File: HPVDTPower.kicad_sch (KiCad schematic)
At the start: 1 part

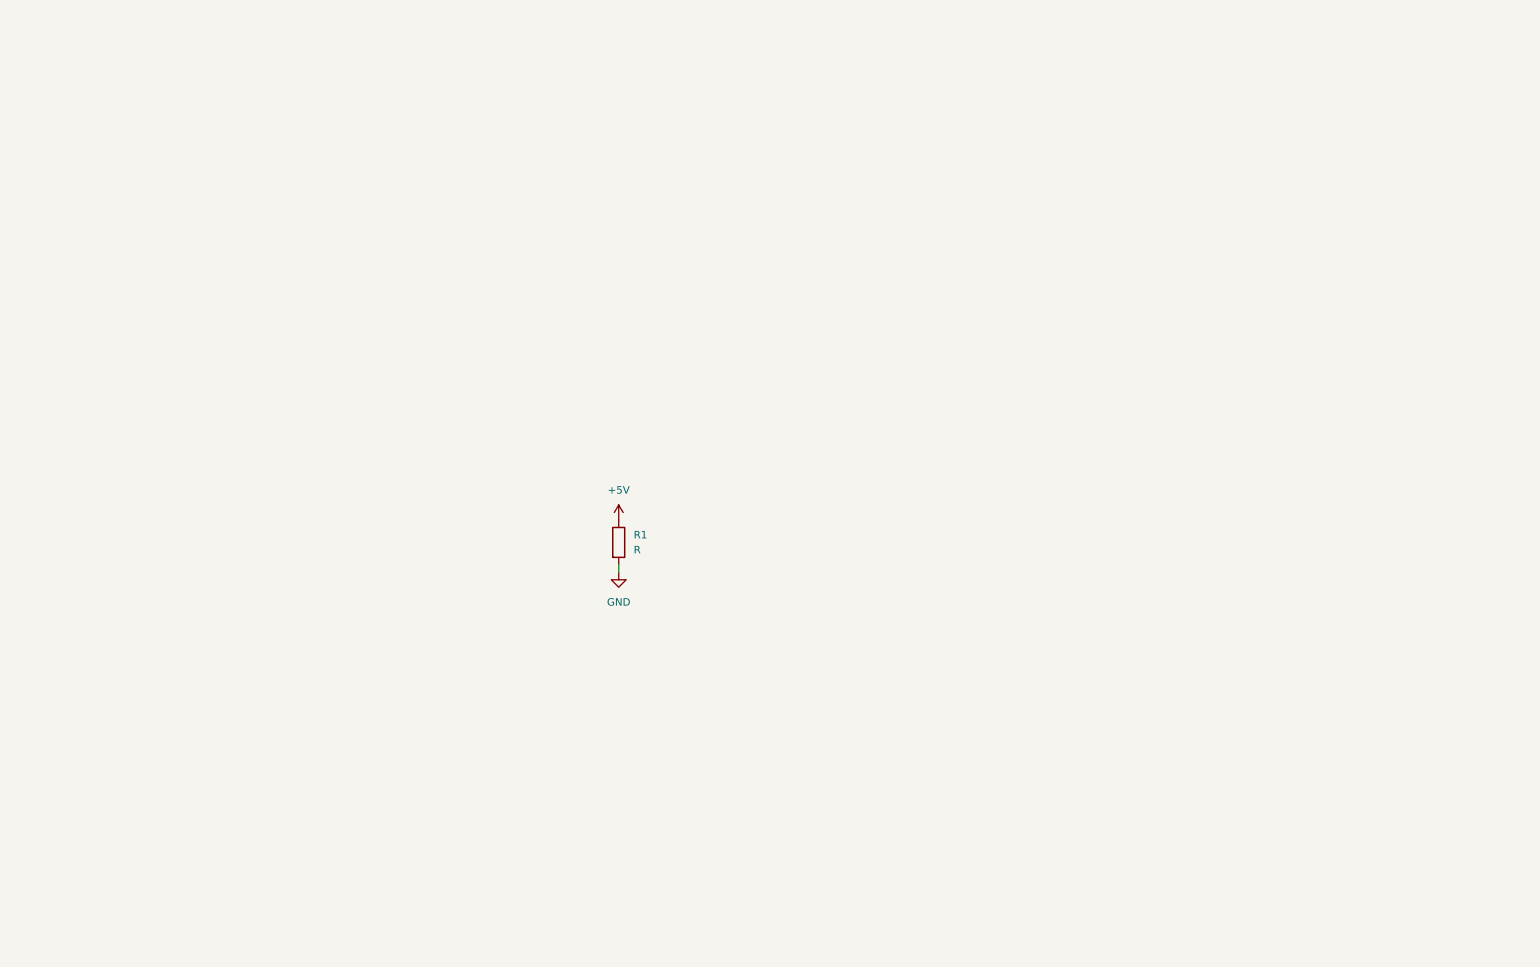
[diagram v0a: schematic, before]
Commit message: Update
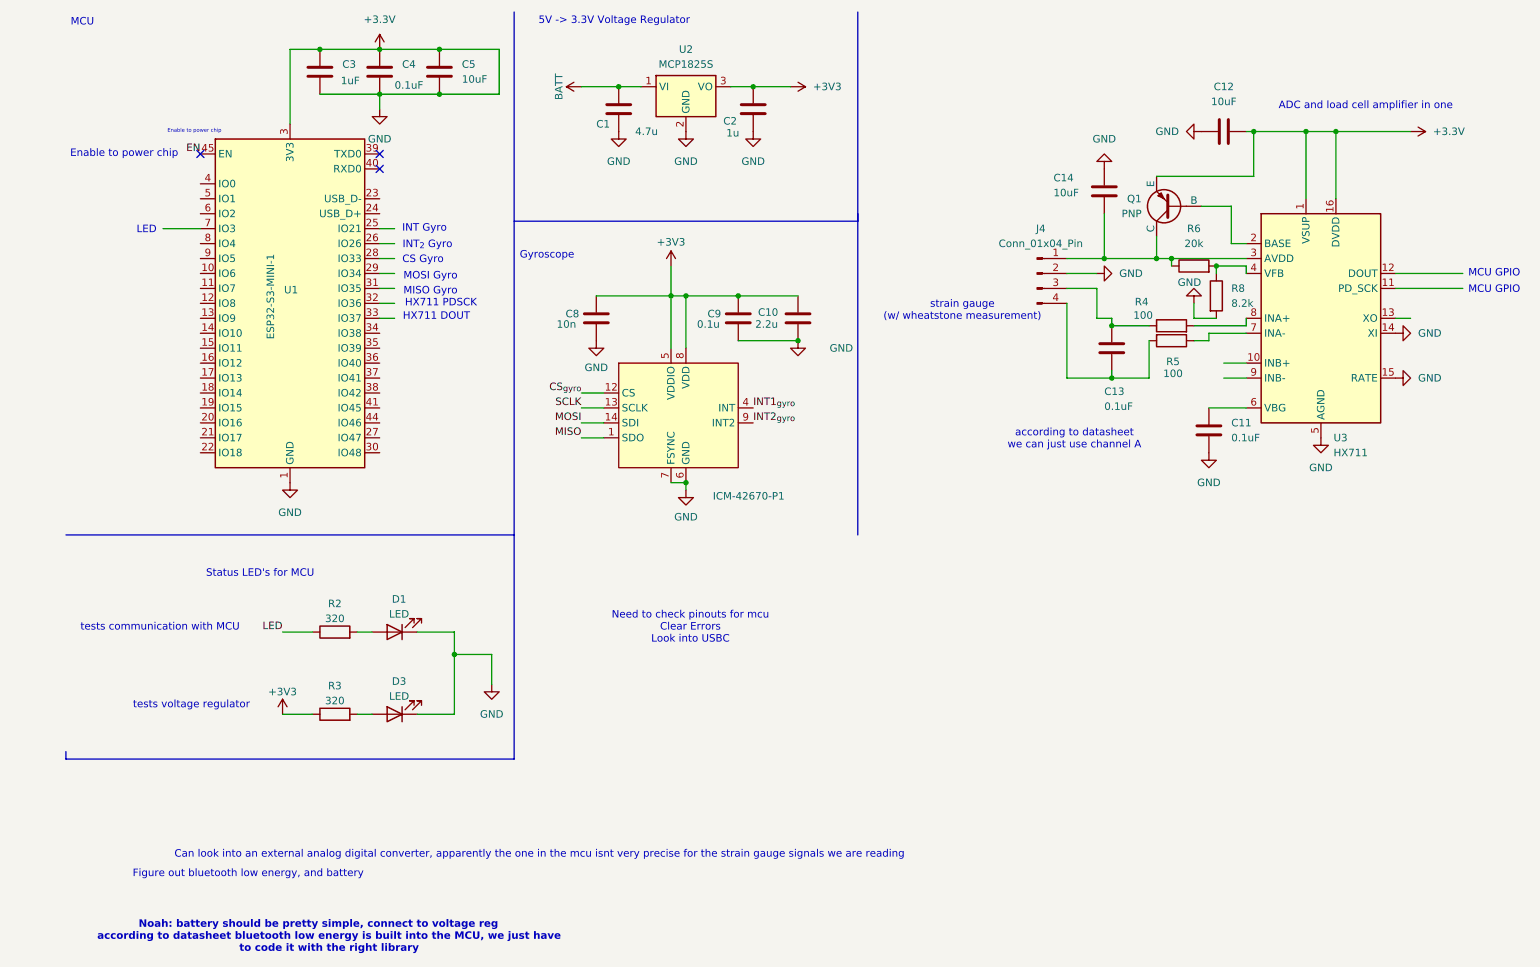
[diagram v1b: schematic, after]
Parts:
- removed R1: R, symbol Device:R
- added C1: 4.7u, Capacitor_SMD:C_0402_1005Metric, symbol Device:C
- added C10: 2.2u, Capacitor_SMD:C_0402_1005Metric, symbol Device:C
- added C11, C13, C4: 0.1uF, symbol Device:C
- added C12, C14, C5: 10uF, symbol Device:C
- added C2: 1u, Capacitor_SMD:C_0402_1005Metric, symbol Device:C
- added C3: 1uF, symbol Device:C
- added C8: 10n, Capacitor_SMD:C_0402_1005Metric, symbol Device:C
- added C9: 0.1u, Capacitor_SMD:C_0402_1005Metric, symbol Device:C
- added D1, D3: LED, LED_SMD:LED_0402_1005Metric, symbol Device:LED
- added ICM-42670-P1: ~, Package_LGA:LGA-14_3x2.5mm_P0.5mm_LayoutBorder3x4y, symbol 0_pwrmtr:ICM-42670-P
- added J4: Conn_01x04_Pin, Connector_JST:JST_EH_S4B-EH_1x04_P2.50mm_Horizontal, symbol Connector:Conn_01x04_Pin
- added Q1: PNP, symbol Simulation_SPICE:PNP
- added R2, R3: 320, Resistor_SMD:R_0402_1005Metric, symbol Device:R
- added R4, R5: 100, symbol Device:R
- added R6: 20k, symbol Device:R
- added R8: 8.2k, symbol Device:R
- added U1: ESP32-S3-MINI-1, RF_Module:ESP32-S2-MINI-1, symbol RF_Module:ESP32-S3-MINI-1
- added U2: MCP1825S, Package_TO_SOT_SMD:SOT-223-3_TabPin2, symbol Regulator_Linear:MCP1825S
- added U3: HX711, Package_SO:SOP-16_3.9x9.9mm_P1.27mm, symbol Analog_ADC:HX711
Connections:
- new net: D1.2 (A), R2.2
- new net: R5.1, U3.7 (INA-)
- new net: C13.2, J4.4 (Pin_4), R5.2
- new net: D3.2 (A), R3.2
- new net: C14.2, J4.1 (Pin_1), Q1.1 (C), R6.1, U3.3 (AVDD)
- new net: C13.1, J4.3 (Pin_3), R4.1
- new net: C11.1, U3.6 (VBG)
- new net: R6.2, R8.1, U3.4 (VFB)
- new net: R4.2, U3.8 (INA+)
- new net: Q1.2 (B), U3.2 (BASE)
- new net +3.3V: C1.1, C10.1, C11.2, C12.1, C12.2, C14.1, C2.1, C3.1, C3.2, C4.1, C4.2, C5.1, C5.2, C8.1, C9.1, D1.1 (K), D3.1 (K), ICM-42670-P1.6 (GND), ICM-42670-P1.7 (FSYNC), J4.2 (Pin_2), Q1.3 (E), R8.2, U1.1 (GND), U1.2 (GND), U1.3 (3V3), U1.42 (GND), U1.43 (GND), U1.46 (GND), U1.47 (GND), U1.48 (GND), U1.49 (GND), U1.50 (GND), U1.51 (GND), U1.52 (GND), U1.53 (GND), U1.54 (GND), U1.55 (GND), U1.56 (GND), U1.57 (GND), U1.58 (GND), U1.59 (GND), U1.60 (GND), U1.61 (GND), U1.62 (GND), U1.63 (GND), U1.64 (GND), U1.65 (GND), U2.2 (GND), U3.1 (VSUP), U3.14 (XI), U3.15 (RATE), U3.16 (DVDD), U3.5 (AGND)
- new net +3V3: C10.2, C2.2, C8.2, C9.2, ICM-42670-P1.5 (VDDIO), ICM-42670-P1.8 (VDD), R3.1, U2.3 (VO)
- new net BATT: C1.2, U2.1 (VI)
- new net CS_{gyro}: ICM-42670-P1.12 (CS)
- new net EN: U1.45 (EN)
- new net INT1_{gyro}: ICM-42670-P1.4 (INT)
- new net INT2_{gyro}: ICM-42670-P1.9 (INT2)
- new net LED: R2.1
- new net MISO: ICM-42670-P1.1 (SDO)
- new net MOSI: ICM-42670-P1.14 (SDI)
- new net SCLK: ICM-42670-P1.13 (SCLK)
- no-connect marks 0 -> 3
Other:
- note added: "5V -> 3.3V Voltage Regulator"
- note added: "ADC and load cell amplifier in one"
- note added: "CS Gyro"
- note added: "Can look into an external analog digital converter, apparently the one in the mcu isnt very precise for the strain gauge signals we are reading"
- note added: "Enable to power chip"
- note added: "Figure out bluetooth low energy, and battery"
- note added: "Gyroscope"
- note added: "HX711 DOUT"
- note added: "HX711 PDSCK"
- note added: "INT Gyro"
- note added: "INT_{2} Gyro"
- note added: "LED"
- note added: "MCU"
- note added: "MCU GPIO"
- note added: "MISO Gyro"
- note added: "MOSI Gyro"
- note added: "Need to check pinouts for mcu Clear Errors Look into USBC"
- note added: "Noah: battery should be pretty simple, connect to voltage reg according to datasheet bluetooth low energy is built into the MCU, we just have to code it with the right library"
- note added: "Status LED's for MCU"
- note added: "according to datasheet we can just use channel A"
- note added: "strain gauge (w/ wheatstone measurement)"
- note added: "tests communication with MCU"
- note added: "tests voltage regulator"
